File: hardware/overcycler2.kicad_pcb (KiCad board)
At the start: 2 copper layers, 215.9 x 152.4 mm, 263 parts, among them IC1 LM13700, IC2 LM13700, IC3 LM13700, P1 LPC_P1, P2 LPC_P2, P3 FT232, P4 PANEL, P5 SDCARD, P6 MIDI_IN, P7 FOOT_IN, P8 AC_IN, P9 AUDIO_OUT, Q1 BC547, SW1 RESET, U1 TLV1543, U10 MCP4922-E/P, U11 SSM2044, U12 MCP4922-E/P, U13 SSM2044, U14 MCP4922-E/P, U15 SSM2044, U16 MCP4922-E/P, U17 SSM2044, U18 MCP4922-E/P, U19 SSM2044, U2 74HCT4051, U20 MCP4922-E/P, U21 SSM2044, U3 LTC1660, U4 LTC1660, U5 TL074, U6 TL074, U7 LM1084IT-5.0/NOPB, U8 LM2990-5.0/NOPB, U9 LM1084IT-3.3/NOPB

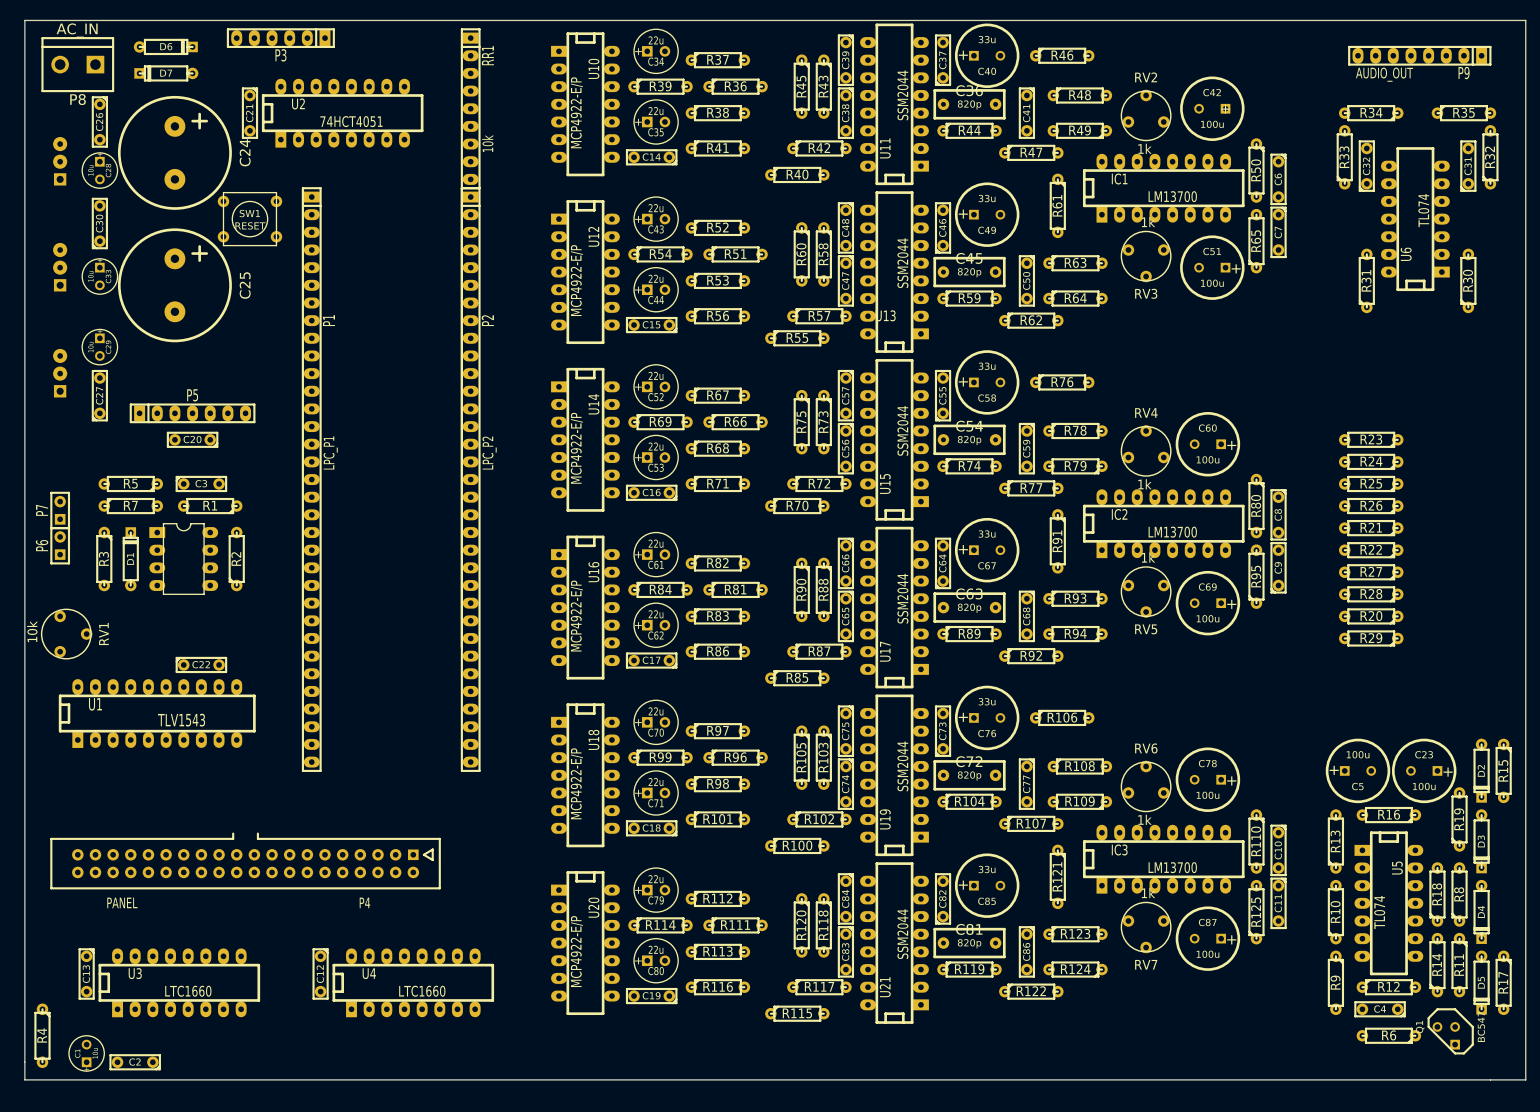
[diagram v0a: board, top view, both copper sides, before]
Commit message: better pcb placement -- sch fixes
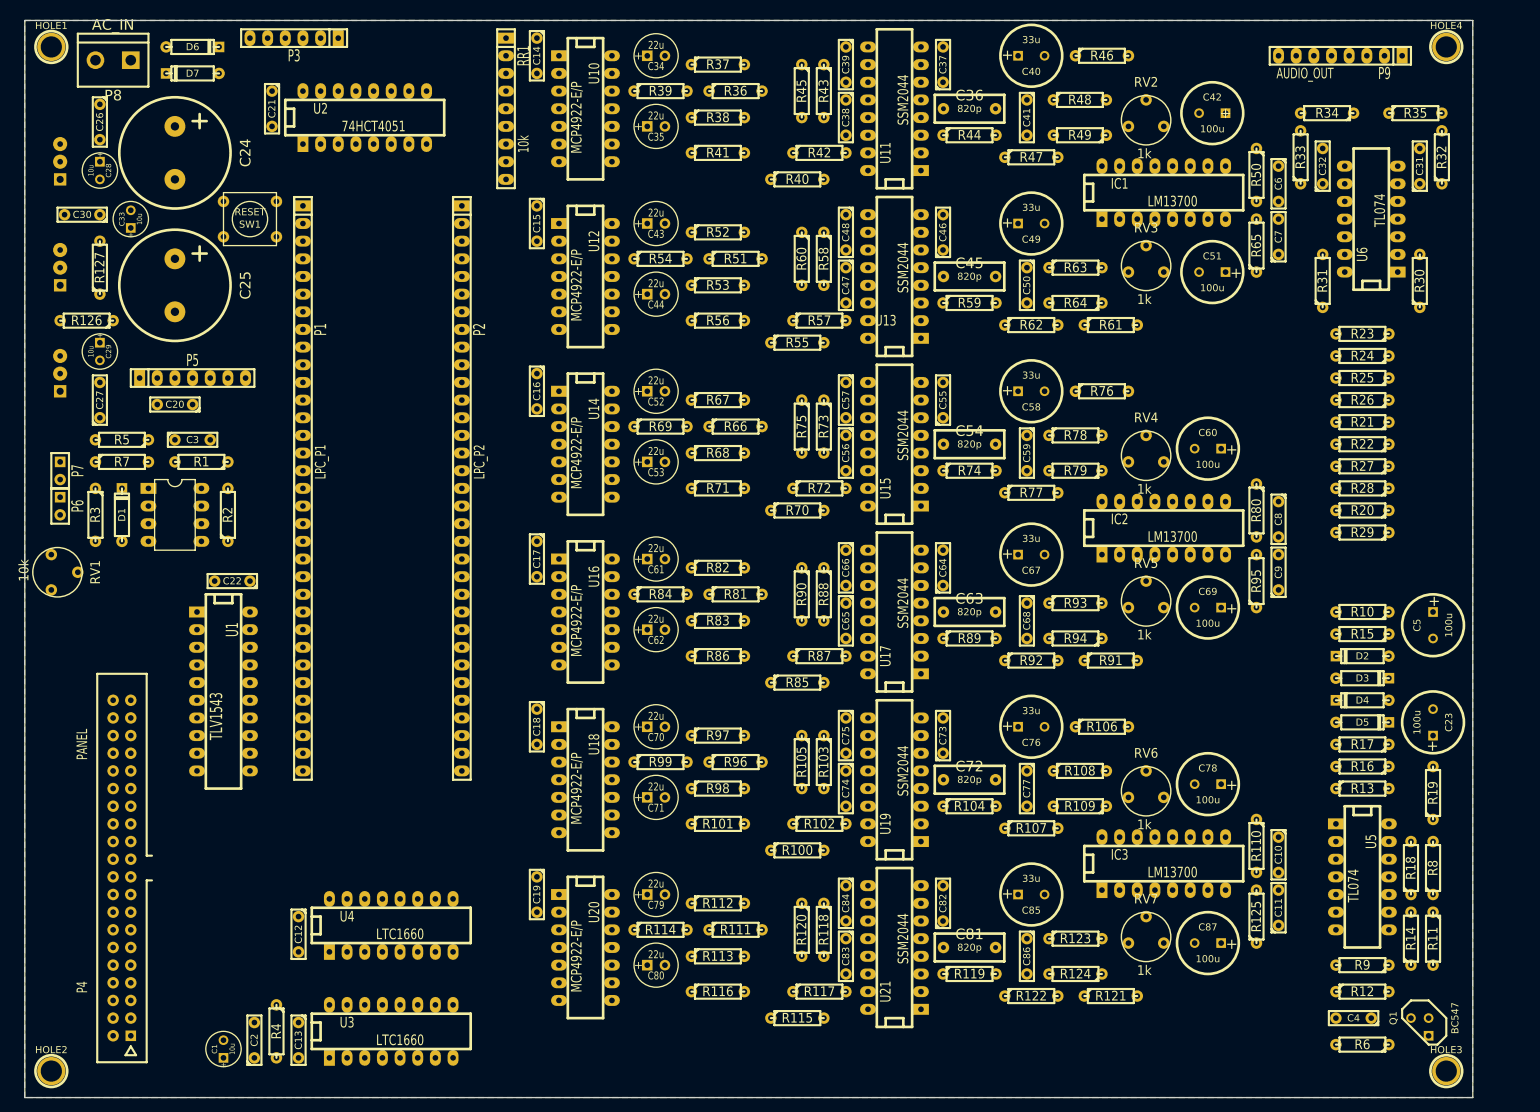
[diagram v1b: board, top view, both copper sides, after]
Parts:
- added HOLE1: P***, 1pin, F.Cu at (29.2, 29.2)
- added HOLE2: P***, 1pin, F.Cu at (29.2, 176.5)
- added HOLE3: P***, 1pin, F.Cu at (229.9, 176.5)
- added HOLE4: P***, 1pin, F.Cu at (229.9, 29.2)
- added R126: 220, R3-LARGE_PADS, F.Cu at (34.3, 68.6)
- added R127: 120, R3-LARGE_PADS, F.Cu at (36.2, 61.0)
- U9: value LM1084IT-3.3/NOPB -> LM1084IT-ADJ/NOPB
- moved R10 43.3 mm to (217.8, 110.5), turned to 180 degrees
- moved D5 41.2 mm to (217.8, 126.4), turned to 0 degrees
- moved R17 39.9 mm to (217.8, 129.5), turned to 180 degrees
- moved D4 35.0 mm to (217.8, 123.2), turned to 180 degrees
- moved R4 33.7 mm to (61.6, 170.8)
- moved C13 31.9 mm to (64.8, 172.1)
- moved U3 31.3 mm to (78.1, 170.8)
- moved D3 29.1 mm to (217.8, 120.0), turned to 0 degrees
- moved R15 28.3 mm to (217.8, 113.7), turned to 180 degrees
- moved D2 23.8 mm to (217.8, 116.8), turned to 180 degrees
- moved C5 23.6 mm to (228.0, 112.4), turned to 270 degrees
- moved C19 22.0 mm to (99.1, 151.1), turned to 270 degrees
- moved C14 22.0 mm to (99.1, 30.5), turned to 270 degrees
- moved C15 22.0 mm to (99.1, 54.6), turned to 270 degrees
- moved C16 22.0 mm to (99.1, 78.7), turned to 270 degrees
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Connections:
- P1 pad 4: N-00000116 -> N-0000060
- P2 pad 21: /KP_1_R1 -> /KP_4_R4
- P2 pad 22: /KP_2_R2 -> /KP_3_R3
- P2 pad 23: /KP_3_R3 -> /KP_2_R2
- P2 pad 24: /KP_4_R4 -> /KP_1_R1
- P4 pad 20: /KP_2_R2 -> /KP_5_C1
- P4 pad 21: /KP_3_R3 -> /KP_2_R2
- P4 pad 22: /KP_4_R4 -> /KP_6_C2
- P4 pad 23: /KP_5_C1 -> /KP_3_R3
- P4 pad 24: /KP_6_C2 -> /KP_7_C3
- P4 pad 25: /KP_7_C3 -> /KP_4_R4
- SW1 pad 1: GND -> N-0000060
- SW1 pad 2: N-00000116 -> GND
- U9 pad 1: GND -> N-0000064
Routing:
- added copper zone on B.Cu, net GND
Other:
- board size 215.9 x 152.4 mm -> 208.3 x 154.9 mm
- net class Default: via_dia 1.016 -> 1.27
- net class pwr2: clearance 0.635 -> 0.4826
